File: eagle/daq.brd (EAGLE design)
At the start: 59.7 x 65.4 mm, 79 parts

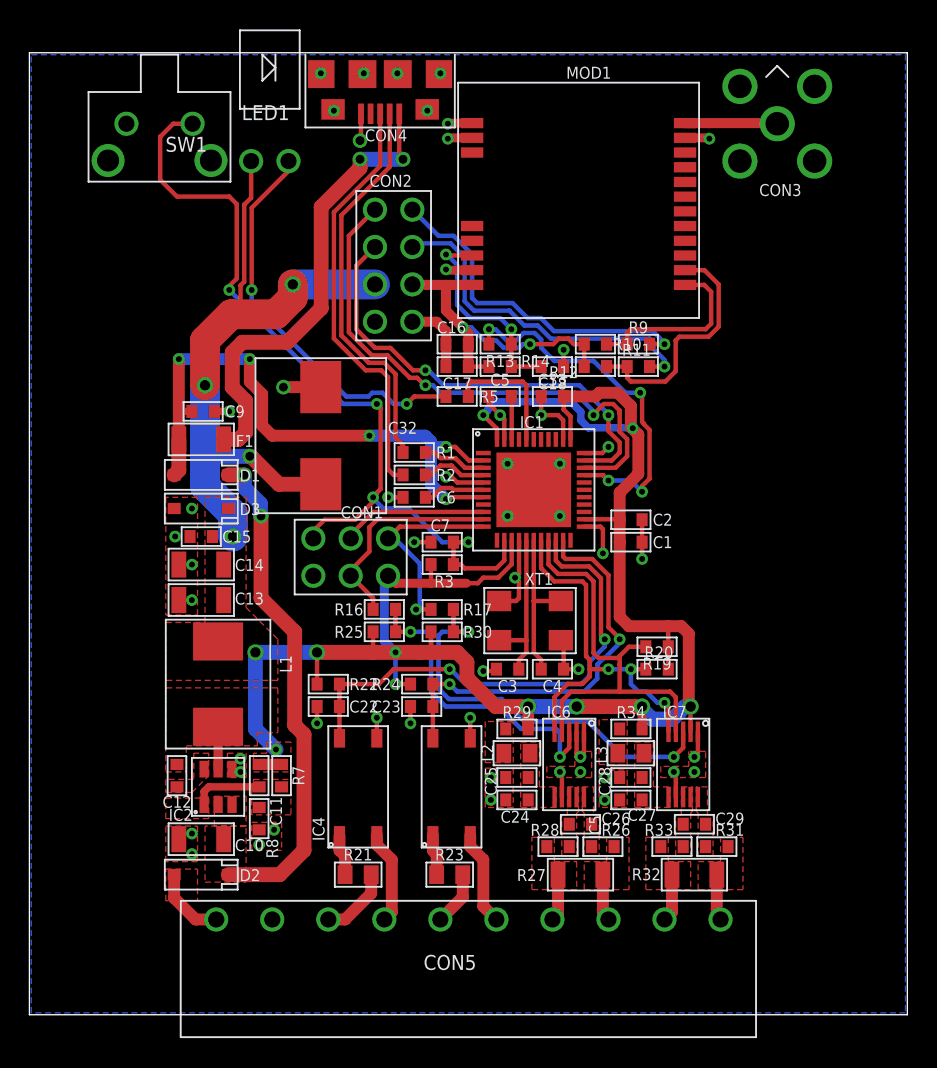
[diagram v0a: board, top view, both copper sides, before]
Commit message: do
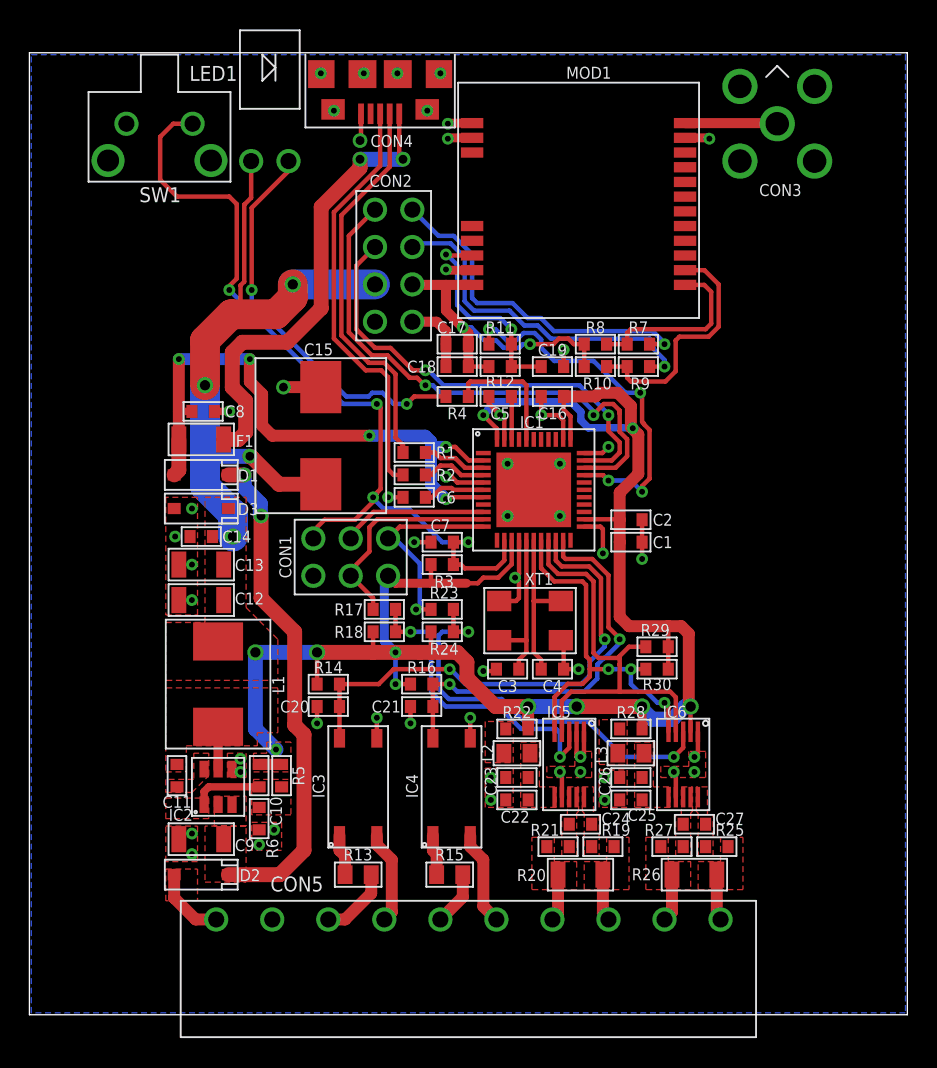
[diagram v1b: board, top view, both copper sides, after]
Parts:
- removed C28, C29, C33, R31, R33, R34: (no value), myparts:0603
- removed C32: (no value), myparts:CAPACITOR-SMD-8
- removed IC7: (no value), myparts:VSSOP-10
- removed R32: (no value), myparts:1206
- added C19, C20, C21, C8, R18, R4, R6: (no value), myparts:0603
- added IC3: (no value), myparts:OPTO-SMD
- added R15: (no value), myparts:0805
- C10, C14, R27: device myparts:1206 -> myparts:0603
- C12, C9, R20, R26: device myparts:0603 -> myparts:1206
- C15: device myparts:0603 -> myparts:CAPACITOR-SMD-8
- IC5: device myparts:OPTO-SMD -> myparts:VSSOP-10
- R13: device myparts:0603 -> myparts:0805
- R21, R23: device myparts:0805 -> myparts:0603
- moved R8 39.5 mm to (38.5, 45.6), turned to 180 degrees
- moved R7 38.1 mm to (41.4, 45.6), turned to 180 degrees
- moved R13 37.3 mm to (22.4, 9.53)
- moved C9 29.1 mm to (11.7, 11.9), turned to 0 degrees
- moved R5 28.4 mm to (17.1, 16.3), turned to 270 degrees
- moved R25 26.9 mm to (46.7, 11.4), turned to 180 degrees
- moved R14 24.5 mm to (20.3, 22.5), turned to 0 degrees
- moved R23 18.0 mm to (28.1, 27.6)
- moved R20 14.9 mm to (37.5, 9.53), turned to 0 degrees
- moved R30 14.8 mm to (42.7, 23.5), turned to 180 degrees
- moved C22 14.3 mm to (33.1, 14.6)
- moved R19 14.1 mm to (39.0, 11.4), turned to 0 degrees
- moved R21 13.7 mm to (35.9, 11.4)
- moved R22 13.2 mm to (33.1, 19.4), turned to 180 degrees
- moved C12 12.1 mm to (11.7, 28.2), turned to 0 degrees
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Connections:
- net GND: now also C12.1, C19.1, C20.1, C21.1, C26.1, C8.1, IC3.3, IC5.1, IC5.2, IC5.7, R6.1; no longer C10.1, C24.1, C27.1, C28.1, C32.1, C33.1, IC5.3, IC6.2, IC7.1, IC7.7, R8.1
- net N$1: now also R4.1; no longer R5.1
- net N$13: now also C18.2, R8.2; no longer C16.2, R14.2
- net N$14: now also R7.1; no longer R9.1
- net N$16: now also R9.1; no longer R11.1
- net N$17: now also C27.1, IC6.8, IC6.9, R27.2; no longer C29.1, IC7.8, IC7.9, R33.2
- net N$2: now also C19.2, R11.1, R12.1; no longer C18.2, R13.1, R14.1
- net N$20: now also IC3.1, R13.2; no longer IC4.1, R21.2
- net N$21: now also C27.2, IC6.10, R25.2; no longer C29.2, IC7.10, R31.2
- net N$22: now also R11.2; no longer R13.2
- net N$23: now also IC5.3, R17.1, R18.2; no longer IC6.3, R16.1, R25.2
- net N$25: now also IC6.3, R23.1, R24.2; no longer IC7.3, R17.1, R30.2
- net N$26: now also R4.2; no longer R5.2
- net N$27: now also R28.2; no longer R34.2
- net N$3: now also R23.2; no longer R17.2
- net N$32: now also C21.2, IC4.4, R16.2; no longer C23.2, IC5.4, R24.2
- net N$33: now also IC4.1, R15.2; no longer IC5.1, R23.2
- net N$35: now also C20.2, IC3.4, R14.2; no longer C22.2, IC4.4, R22.2
- net N$40: now also R25.1, R26.1; no longer R31.1, R32.1
- net N$42: now also C25.2, C26.2, IC6.6; no longer C27.2, C28.2, IC7.6
- net N$49: now also IC4.2; no longer IC5.2
- net N$50: now also IC3.2; no longer IC4.2
- net N$55: now also R15.1; no longer R23.1
- net N$57: now also C9.2; no longer C10.2
- net N$59: now also R20.1, R21.2; no longer R27.1, R28.2
- net N$6: now also R7.2, R8.1; no longer R10.1, R9.2
- net N$65: now also C11.2; no longer C12.2
- net N$66: now also C11.1; no longer C12.1
- net N$68: now also C24.2, IC5.10, R19.1; no longer C26.2, IC6.10, R26.1
- net N$69: now also C24.1, IC5.8, IC5.9, R21.1; no longer C26.1, IC6.8, IC6.9, R28.1
- net N$7: now also R10.1, R9.2; no longer R11.2, R12.1
- net N$71: now also R22.2; no longer R29.2
- net N$72: now also C10.1, R5.2, R6.2; no longer C11.1, R7.2, R8.2
- net N$73: now also IC5.5, R30.2; no longer IC7.5, R20.2
- net N$77: now also C22.2, C23.2, IC5.6; no longer C24.2, C25.2, IC6.6
- net N$79: now also IC5.4, R29.2; no longer IC7.4, R19.2
- net N$8: now also R26.2, R27.1; no longer R32.2, R33.1
- net N$81: now also R19.2, R20.2; no longer R26.2, R27.2
- net N$85: now also R13.1; no longer R21.1
- net N$9: now also R17.2; no longer R16.2
- net UVCC: now also C8.2; no longer C9.2
- net VCC: now also C10.2, C12.2, C16.2, IC6.2, R14.1, R16.1, R18.1, R28.1, R5.1; no longer C11.2, C32.2, C33.2, IC7.2, R19.1, R20.1, R25.1, R34.1, R7.1
